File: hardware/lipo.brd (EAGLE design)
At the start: 33.5 x 34.6 mm, 62 parts, among them IC1 4066D, IC2 4066D, J1 MICRO_USB_B_HIROSE_ZX62-B-5PA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, Q1 IRLML6402, SW1 TVAF06-A020B-R, U1 LT6106CS5#PBF, U2 NJM12888F, U3 MCP73831, U5 TCK106AF,LF, X1 FA-238

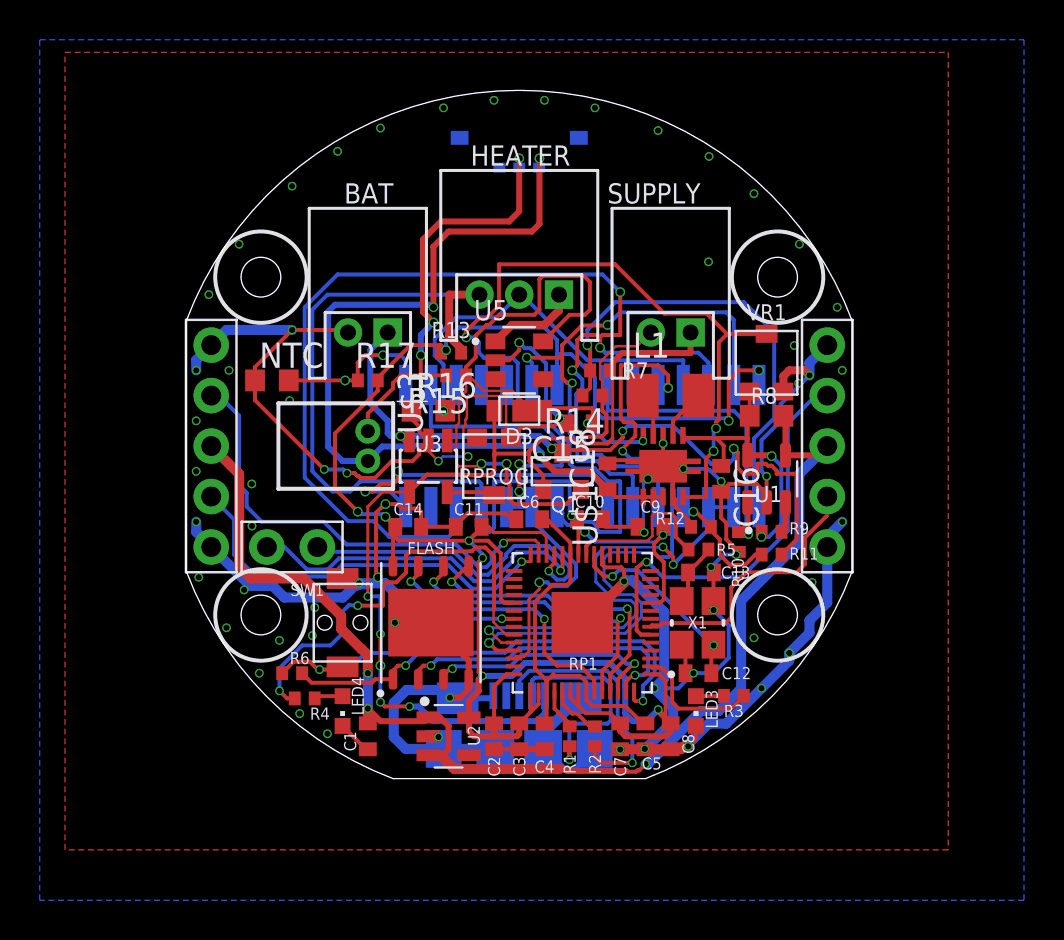
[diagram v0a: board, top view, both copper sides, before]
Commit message: 回路微修正
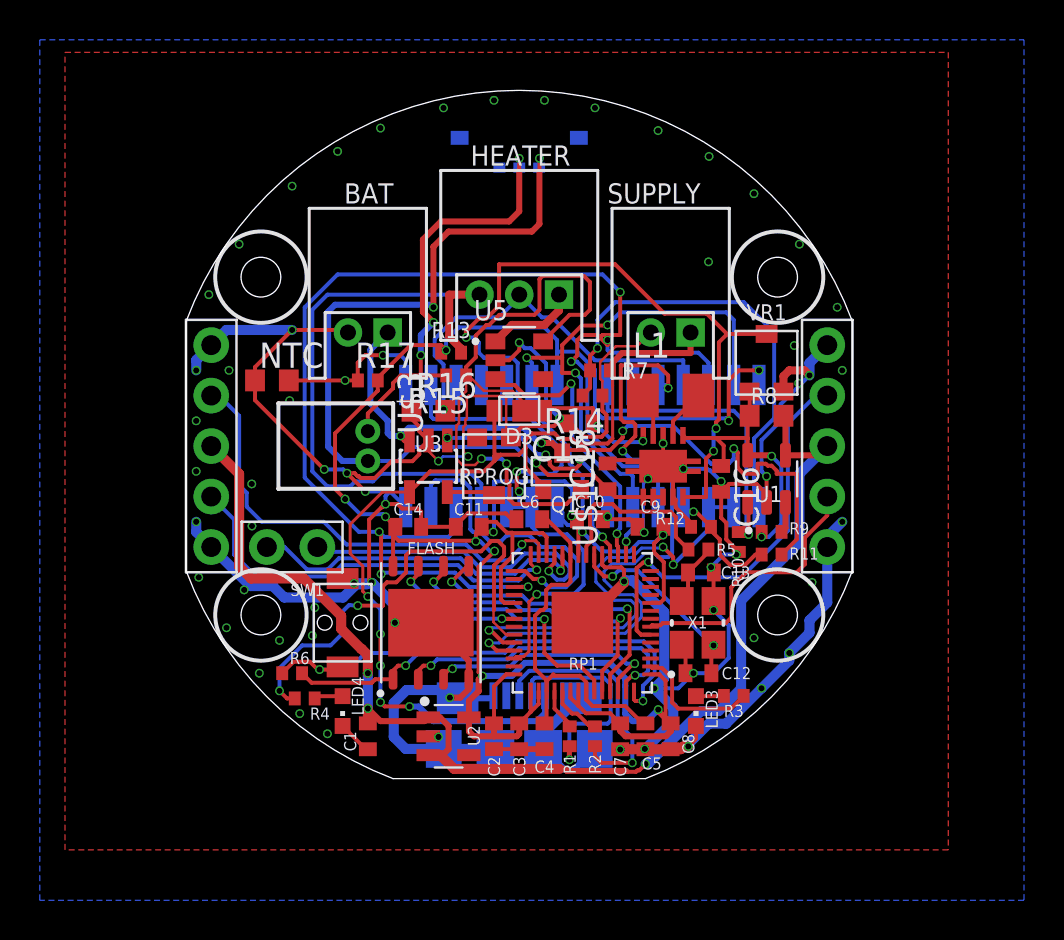
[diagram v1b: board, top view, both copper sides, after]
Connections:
- removed net N$5: J1.ID
- removed net VSS: IC1.7, IC2.7
- net ADC_SEL1: now also RP1.16
- net ADC_SEL2: now also RP1.31
- net ADC_SEL3: now also RP1.29
- net CHARGE: now also RP1.18
- net GND: now also IC1.7, IC2.7
- net HEATER: now also RP1.17
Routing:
- net VSS: track 16.4 -> 0.00 mm, vias 2 -> 0
- net ADC_SEL3: track 0.00 -> 16.2 mm, vias 0 -> 1
- net HEATER: track 0.00 -> 14.1 mm, vias 0 -> 2
- net CHARGE: track 0.00 -> 13.2 mm, vias 0 -> 4
- net ADC_SEL2: track 59.8 -> 69.9 mm, vias 3 -> 6
- net GND: track 212.1 -> 216.9 mm, vias 69 -> 71
- net V+_V: track 48.9 -> 44.1 mm
- net ADC_SEL1: track 27.1 -> 28.9 mm, vias 3 -> 4
- net ADC2_IN: track 26.9 -> 28.2 mm
- net LED1: track 21.9 -> 23.2 mm
- net ADC1_IN: track 35.1 -> 34.2 mm
- net VPP: track 49.9 -> 50.7 mm
- net XOUT1: track 8.19 -> 9.01 mm
- net SWCLK: track 18.0 -> 17.2 mm
- net SWD: track 17.1 -> 16.4 mm
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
